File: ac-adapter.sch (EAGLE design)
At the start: 45 parts, among them IC2 TL431, Q1 300V5A, Q2 300V5A, Q3 TLP621-1, T1 COMMON_FILTER-SU10VFC, T2 TRANSFORMAER_FLYBACK-PQ2620, T3 COMMON_FILTER-SMALL

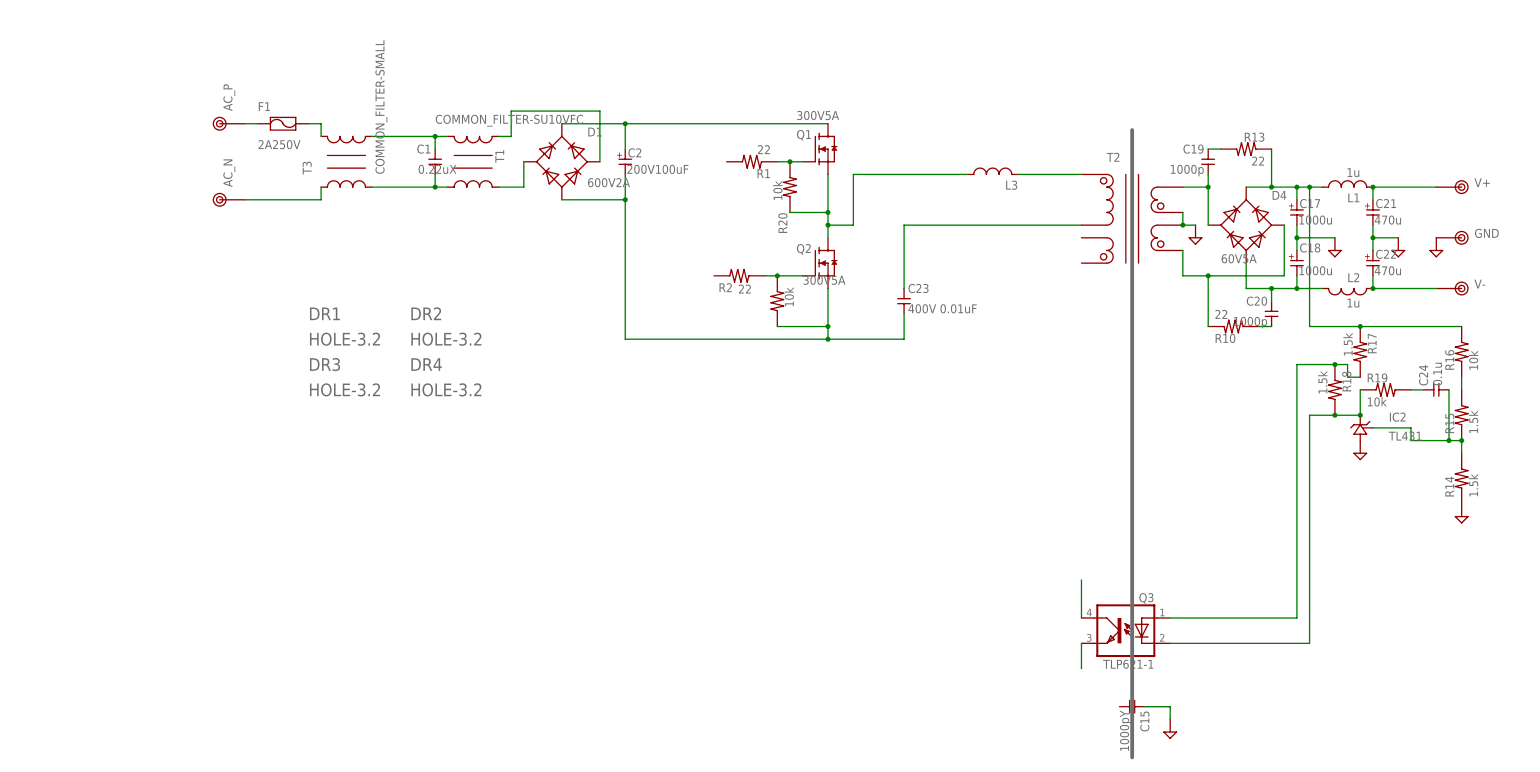
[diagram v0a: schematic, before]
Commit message: 定数決まらん
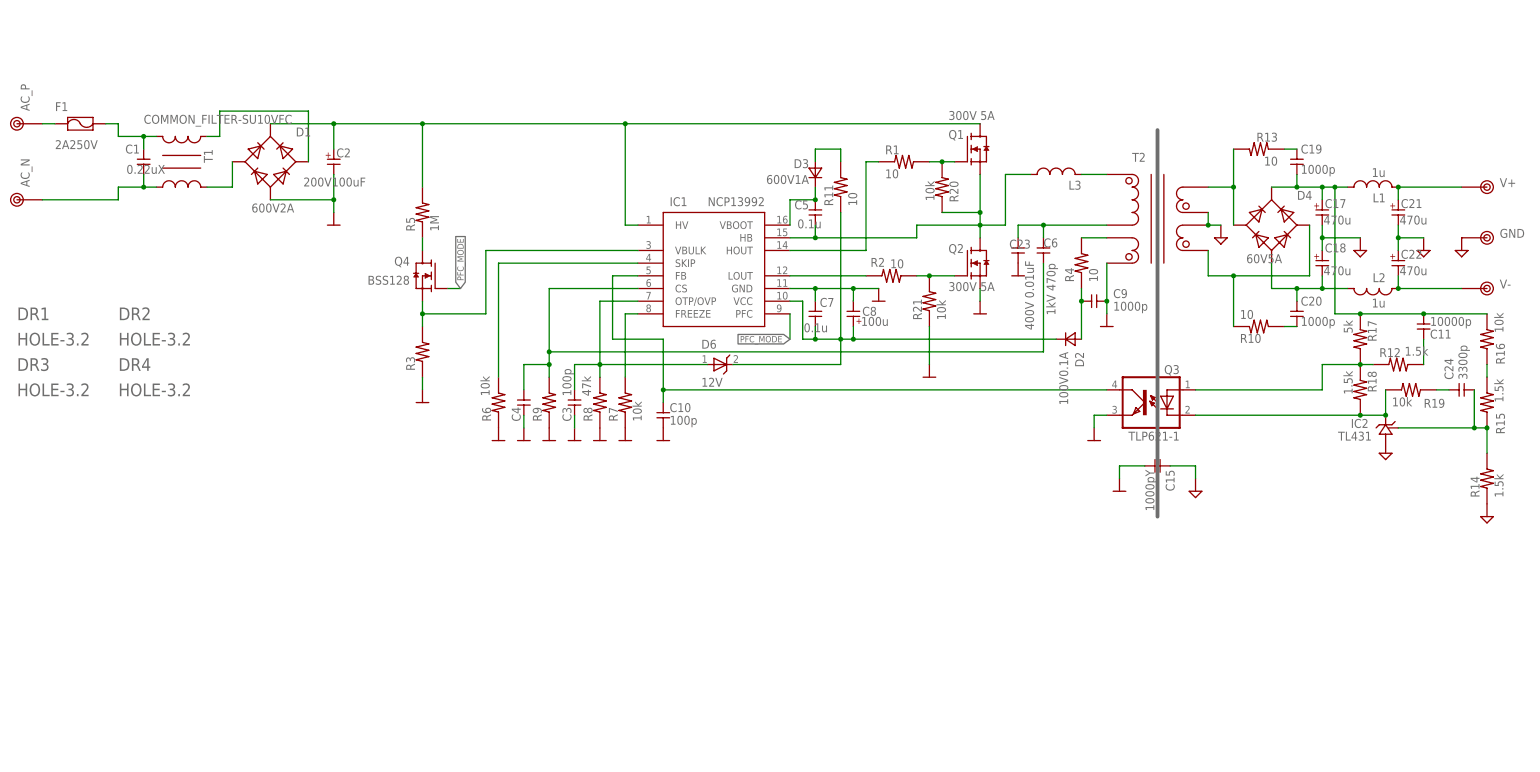
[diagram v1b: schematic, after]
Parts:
- removed T3: COMMON_FILTER-SMALL, my_rcl:COMMON_FILTER-SMALL
- added C10, C3: 100p, my_rcl:C-1608
- added C11: 10000p, my_rcl:C-1608
- added C4: (no value), my_rcl:C-1608
- added C5, C7: 0.1u, my_rcl:C-1608
- added C6: 1kV 470p, my_rcl:C-5
- added C8: 100u, my_rcl:CPOLE2.5-6.5
- added C9: 1000p, my_rcl:C-1608
- added D2: 100V0.1A, my_rcl:DIODE-1N4148W
- added D3: 600V1A, my_rcl:DIODE-7
- added D6: 12V, my_rcl:ZENER-SMD
- added IC1: NCP13992, my_ic:NCP13992
- added Q4: BSS128, my_ic:NMOS-SMD
- added R11, R4: 10, my_rcl:R-1608
- added R12: 1.5k, my_rcl:R-1608
- added R3, R9: (no value), my_rcl:R-1608
- added R5: 1M, my_rcl:R-7.5
- added R6, R7: 10k, my_rcl:R-1608
- added R8: 47k, my_rcl:R-1608
- C17, C18: value 1000u -> 470u
- C2: device my_rcl:CPOLE7.5-16A -> my_rcl:CPOLE7.5-16A2
- C24: value 0.1u -> 3300p
- Q1, Q2: value 300V5A -> 300V 5A
- R1, R2: value 22 -> 10; device my_rcl:R-7.5 -> my_rcl:R-2012
- R10, R13: value 22 -> 10; device my_rcl:R-2.5 -> my_rcl:R-2012
- R17: value 1.5k -> 5k
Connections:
- removed net N$30: T3.1, TP2.1
- removed net N$31: F1.P$2, T3.4
- removed net N$43: Q3.EMIT
- removed net N$44: C2.2, C23.2, D1.V-, Q2.S, R21.1
- new net N$12: IC1.FREEZE, R7.2
- new net N$13: C3.1, D6.A, IC1.OTP/OVP, R8.2
- new net N$14: C4.1, C6.2, IC1.CS, R9.2
- new net N$15: IC1.SKIP, R6.2
- new net N$16: IC1.HOUT, R1.1
- new net N$17: IC1.LOUT, R2.2
- new net N$18: C5.1, D3.K, IC1.VBOOT
- new net N$19: IC1.VBULK, Q4.S, R3.2
- new net N$20: C10.1, IC1.FB, Q3.COL
- new net N$21: Q4.D, R5.1
- new net N$23: C11.1, R12.2
- new net N$24: C9.1, D2.A, R4.1
- new net N$25: D3.A, R11.2
- new net PFC_MODE: IC1.PFC, Q4.G
- new net PGND: C10.2, C15.2, C2.2, C23.2, C3.2, C4.2, C7.2, C8.2, C9.2, D1.V-, IC1.GND, Q2.S, Q3.EMIT, R21.1, R3.1, R6.1, R7.1, R8.1, R9.1, T2.L2_P
- new net VCC: C7.1, C8.1, D2.K, D6.C, IC1.VCC, R11.1
- net N$1: now also F1.P$2; no longer T3.3
- net N$2: now also R1.2; no longer R1.1
- net N$22: now also R4.2, T2.L2_N; no longer Q3.COL
- net N$26: now also TP2.1; no longer T3.2
- net N$3: now also R13.1; no longer R13.2
- net N$34: now also R12.1
- net N$35: now also R13.2; no longer C19.2
- net N$40: now also C11.2, C19.2; no longer R13.1
- net N$8: now also C6.1
- net SW: now also C5.2, IC1.HB
- net VH: now also IC1.HV, R5.2
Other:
- moved on the sheet: C1, C15, C17, C18, C19, C2, C20, C21, C22, C23, C24, D1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
